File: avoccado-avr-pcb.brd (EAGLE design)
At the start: 17.8 x 40.3 mm, 30 parts, among them IC1 MCP1703CB, IC5 ATMEGA328P-20MU, Q1 #MHz, Q2 MOSFET-NCHANNEL2N7002PW, U1 ATMEGA328P, U2 MCP73831, X1 Micro USB

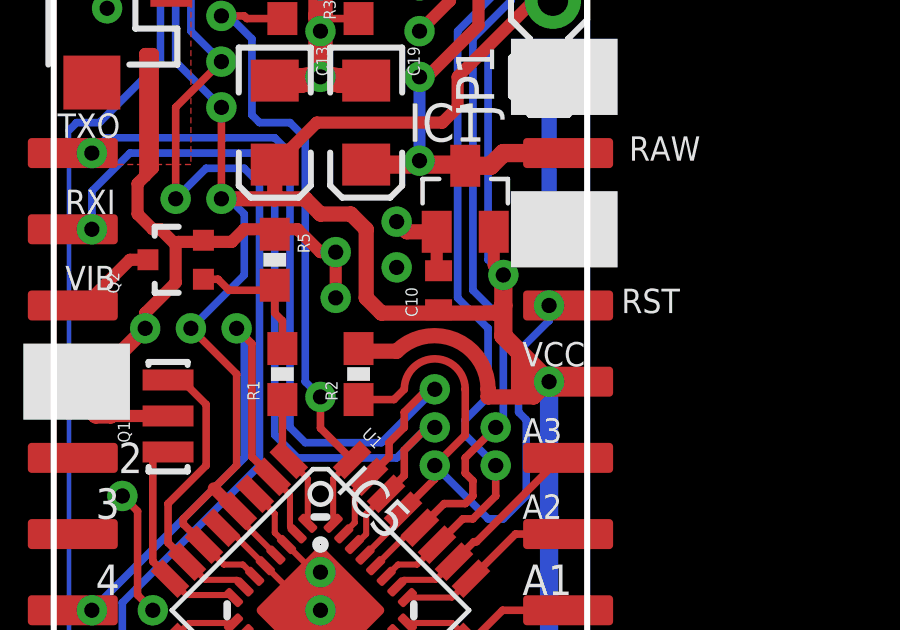
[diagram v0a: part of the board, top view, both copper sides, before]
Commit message: minor corrections
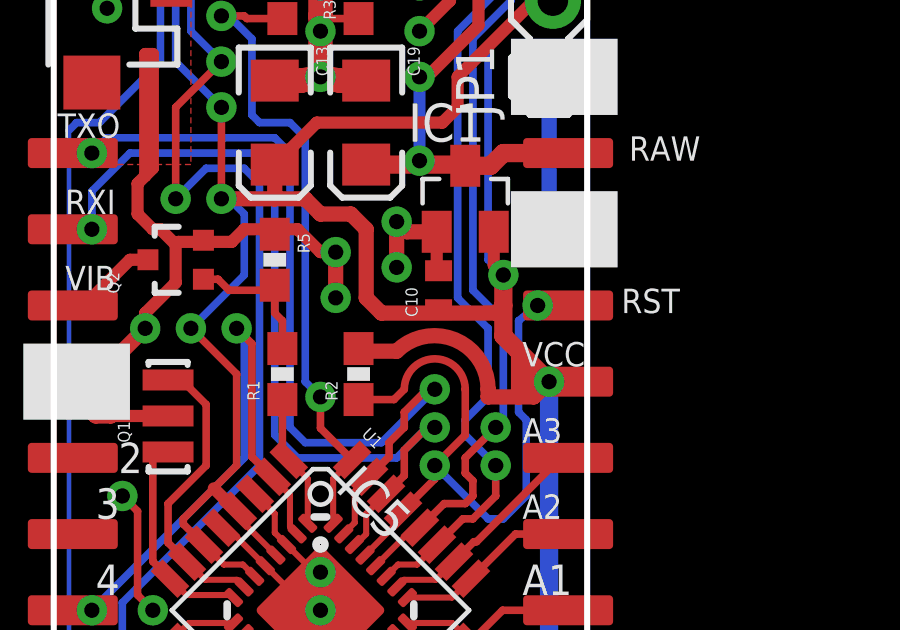
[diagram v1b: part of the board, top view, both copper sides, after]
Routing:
- net GND: track 99.2 -> 100.7 mm
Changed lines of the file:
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@@
 <layer number="14" name="Route14" color="1" fill="6" visible="no" active="no"/>
 <layer number="15" name="Route15" color="4" fill="6" visible="no" active="no"/>
-<layer number="16" name="Bottom" color="1" fill="1" visible="no" active="yes"/>
+<layer number="16" name="Bottom" color="1" fill="1" visible="yes" active="yes"/>
 <layer number="17" name="Pads" color="14" fill="1" visible="yes" active="yes"/>
 <layer number="18" name="Vias" color="14" fill="1" visible="yes" active="yes"/>
@@
 </layers>
 <board>
+<description>Avoccado-avr controller</description>
 <plain>
 <wire x1="8.89" y1="52.07" x2="8.89" y2="11.811" width="0.2032" layer="20"/>
@@
 <wire x1="17.78" y1="37.338" x2="17.018" y2="38.1" width="0.4064" layer="1"/>
 <wire x1="17.018" y1="38.1" x2="16.09" y2="38.1" width="0.4064" layer="1"/>
-<wire x1="18.288" y1="37.338" x2="18.288" y2="35.814" width="0.4064" layer="1"/>
 <via x="18.288" y="35.814" extent="1-16" drill="0.508" diameter="1.016"/>
 <via x="10.668" y="13.97" extent="1-16" drill="0.508" diameter="1.016"/>
@@
 <via x="11.176" y="29.21" extent="1-16" drill="0.508" diameter="1.016"/>
 <wire x1="11.684" y1="28.702" x2="11.176" y2="29.21" width="0.254" layer="1"/>
+<wire x1="20.32" y1="36.83" x2="20.32" y2="38.354" width="0.508" layer="1"/>
 <wire x1="10.16" y1="33.02" x2="9.525" y2="33.02" width="0" layer="19" extent="1-1"/>
 <wire x1="25.4" y1="38.1" x2="21.656" y2="38.016" width="0" layer="19" extent="1-1"/>
+<wire x1="18.288" y1="35.814" x2="18.288" y2="37.338" width="0.508" layer="1"/>
+<wire x1="18.288" y1="37.338" x2="25.4" y2="38.1" width="0" layer="19" extent="1-16"/>
 </signal>
 <signal name="AREF">
@@
 <contactref element="U1" pad="29"/>
 <contactref element="JP3" pad="3"/>
-<wire x1="26.035" y1="35.56" x2="25.4" y2="35.56" width="0.254" layer="1"/>
-<via x="25.4" y="35.56" extent="1-16" drill="0.508" diameter="1.016"/>
+<wire x1="26.035" y1="35.56" x2="25.019" y2="35.56" width="0.254" layer="1"/>
+<via x="25.019" y="35.56" extent="1-16" drill="0.508" diameter="1.016"/>
 <wire x1="23.368" y1="28.448" x2="23.876" y2="28.448" width="0.254" layer="16"/>
 <wire x1="23.876" y1="28.448" x2="24.638" y2="29.21" width="0.254" layer="16"/>
 <wire x1="24.638" y1="29.21" x2="24.638" y2="31.75" width="0.254" layer="16"/>
 <wire x1="24.638" y1="31.75" x2="24.384" y2="32.004" width="0.254" layer="16"/>
-<wire x1="24.384" y1="32.004" x2="24.384" y2="34.036" width="0.254" layer="16"/>
-<wire x1="24.384" y1="34.036" x2="25.4" y2="35.052" width="0.254" layer="16"/>
-<wire x1="25.4" y1="35.052" x2="25.4" y2="35.56" width="0.254" layer="16"/>
+<wire x1="24.384" y1="32.004" x2="24.384" y2="35.052" width="0.254" layer="16"/>
+<wire x1="24.384" y1="35.052" x2="25.019" y2="35.56" width="0.254" layer="16"/>
 <wire x1="20.53248125" y1="28.71816875" x2="21.59" y2="29.7756875" width="0.254" layer="1"/>
 <wire x1="21.59" y1="29.7756875" x2="21.59" y2="30.226" width="0.254" layer="1"/>
